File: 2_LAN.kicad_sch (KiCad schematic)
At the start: 56 parts, among them U1 LAN9514, U5 M93C86-WMN6TP, X1 25MHz

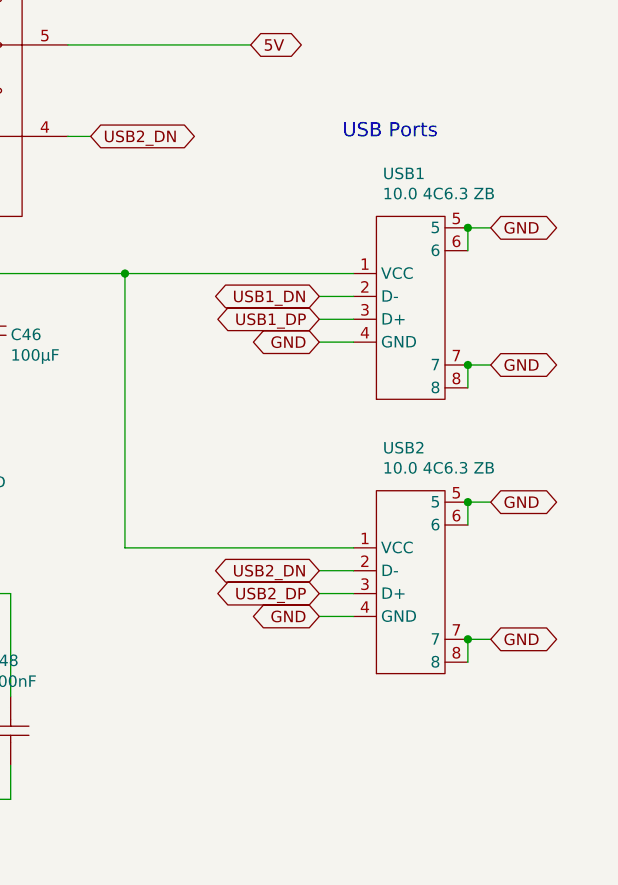
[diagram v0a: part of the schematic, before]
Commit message: switch to vertical USB
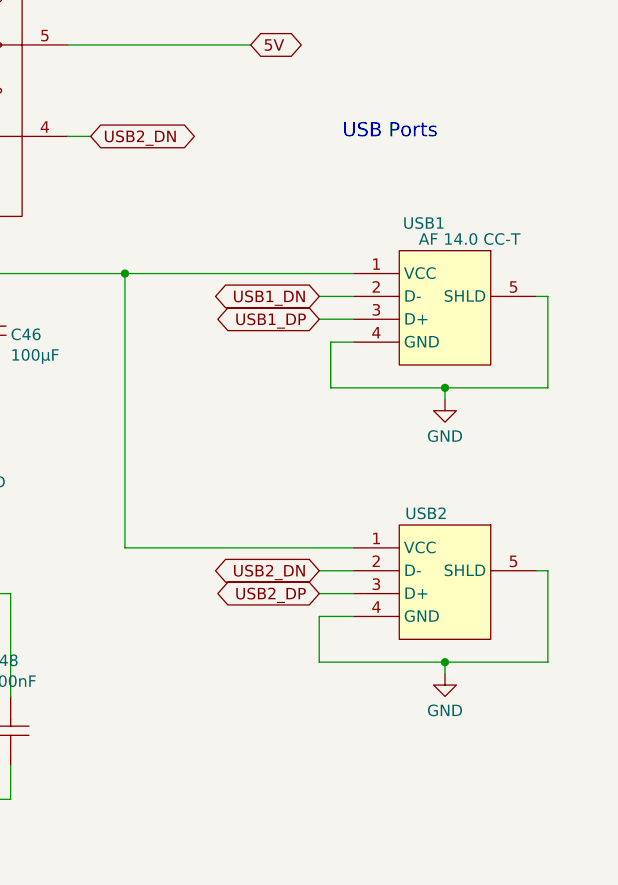
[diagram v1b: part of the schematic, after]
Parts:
- USB1, USB2: value 10.0 4C6.3 ZB -> AF 14.0 CC-T; footprint x1-expander:USB-TH_10.0-4C6.3-ZB -> x1-expander:USB-A-TH_AF14.0CC-T; symbol x1-expander:10.0 4C6.3 ZB -> x1-expander:AF14.0CC-T; LCSC C6386909 -> C456020; LCSC Part (none) -> C456020; Supplier Part C6386909 -> C456020
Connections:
- net GND: no longer USB1.6, USB1.7, USB1.8, USB2.6, USB2.7, USB2.8
